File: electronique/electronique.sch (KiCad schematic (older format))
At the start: 35 parts, among them J1 Conn_02x07_Odd_Even, J10 PHOTOD3, J11 PHOTOD4, J12 Ultrason 3, J13 Moteur 2, J14 Moteur 1, J2 Conn_01x02, J3 Camera, J4 TOF1, J5 Conn_01x06, J6 Ultrason 1, J7 PHOTOD1, J8 PHOTOD2, J9 Ultrason 2, U1 STM32L451RETx, U2 LD1117S50TR_SOT223, U3 LD1117S33TR_SOT223, U4 LB1930MC-AH, U5 LB1930MC-AH, Y1 LFXTAL003240

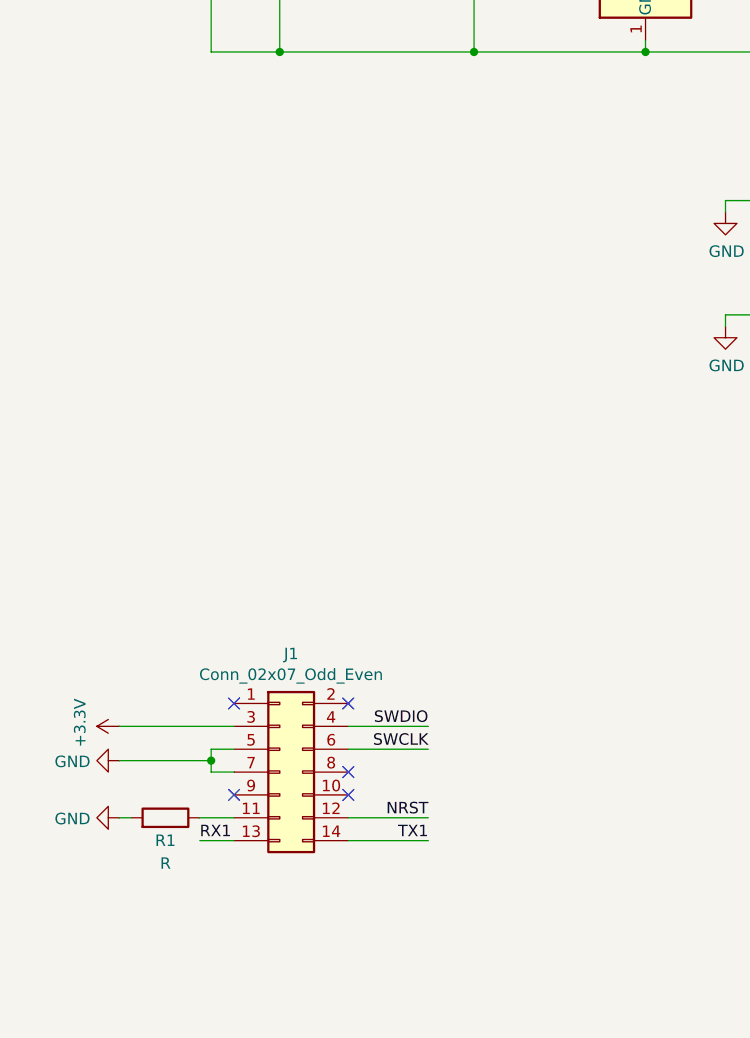
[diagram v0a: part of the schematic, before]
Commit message: Schema mis a jour pour la seance de projet
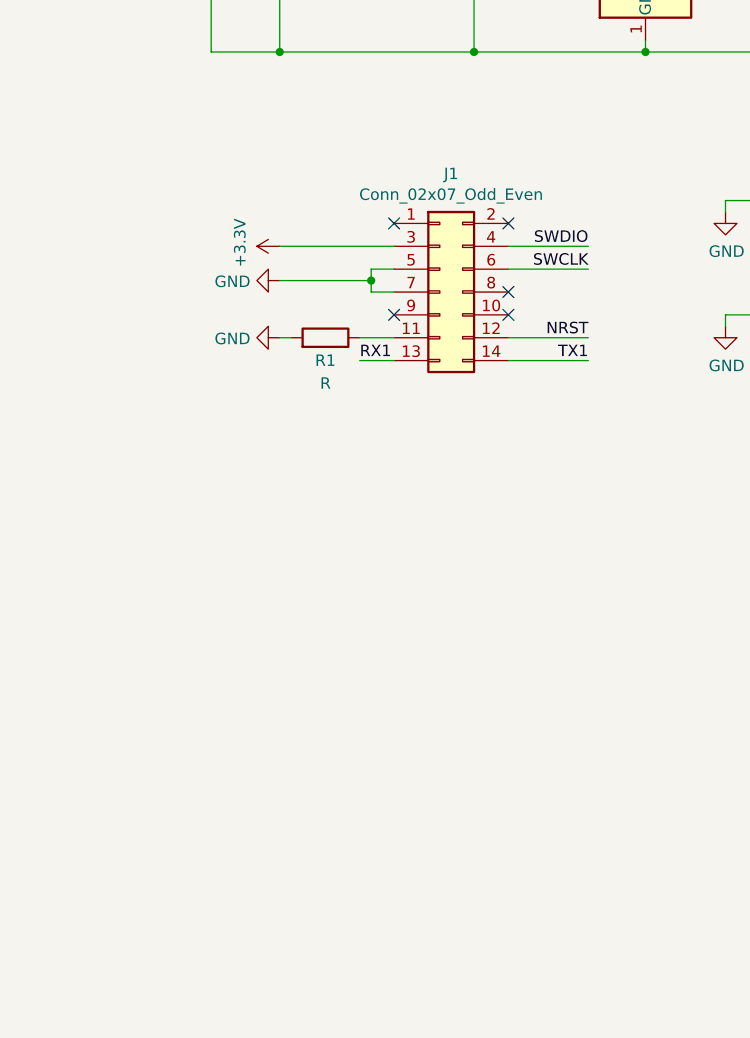
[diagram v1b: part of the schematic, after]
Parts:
- C1, C2: footprint (none) -> Capacitor_SMD:C_0805_2012Metric_Pad1.15x1.40mm_HandSolder
- R8, R9: footprint (none) -> Resistor_THT:R_Axial_DIN0207_L6.3mm_D2.5mm_P7.62mm_Horizontal
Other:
- moved on the sheet: J1, R1
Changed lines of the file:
@@
 EESchema Schematic File Version 4
-EELAYER 30 0
+LIBS:electronique-cache
+EELAYER 29 0
 EELAYER END
 $Descr A4 11693 8268
@@
 F 0 "C1" V 4052 2300 50  0000 C CNN
 F 1 "C" V 3961 2300 50  0000 C CNN
-F 2 "" H 3838 2150 50  0001 C CNN
+F 2 "Capacitor_SMD:C_0805_2012Metric_Pad1.15x1.40mm_HandSolder" H 3838 2150 50  0001 C CNN
 F 3 "~" H 3800 2300 50  0001 C CNN
 	1    3800 2300
@@
 F 0 "C2" V 3548 2800 50  0000 C CNN
 F 1 "C" V 3639 2800 50  0000 C CNN
-F 2 "" H 3838 2650 50  0001 C CNN
+F 2 "Capacitor_SMD:C_0805_2012Metric_Pad1.15x1.40mm_HandSolder" H 3838 2650 50  0001 C CNN
 F 3 "~" H 3800 2800 50  0001 C CNN
 	1    3800 2800
@@
 L Connector_Generic:Conn_02x07_Odd_Even J1
 U 1 1 615F66B1
-P 1550 4800
-F 0 "J1" H 1600 5317 50  0000 C CNN
-F 1 "Conn_02x07_Odd_Even" H 1600 5226 50  0000 C CNN
-F 2 "FTSH:SAMTEC_FTSH-107-01-L-DV-K-A" H 1550 4800 50  0001 C CNN
-F 3 "~" H 1550 4800 50  0001 C CNN
-	1    1550 4800
+P 2250 2700
+F 0 "J1" H 2300 3217 50  0000 C CNN
+F 1 "Conn_02x07_Odd_Even" H 2300 3126 50  0000 C CNN
+F 2 "FTSH:SAMTEC_FTSH-107-01-L-DV-K-A" H 2250 2700 50  0001 C CNN
+F 3 "~" H 2250 2700 50  0001 C CNN
+	1    2250 2700
 	1    0    0    -1
 $EndComp
@@
 	1    0    0    -1
 $EndComp
-NoConn ~ 1350 4500
-NoConn ~ 1850 4500
-NoConn ~ 1850 4800
-NoConn ~ 1850 4900
-NoConn ~ 1350 4900
+NoConn ~ 2050 2400
+NoConn ~ 2550 2400
+NoConn ~ 2550 2700
+NoConn ~ 2550 2800
+NoConn ~ 2050 2800
 $Comp
 L power:GND #PWR0106
 U 1 1 6161C108
-P 850 4750
-F 0 "#PWR0106" H 850 4500 50  0001 C CNN
-F 1 "GND" V 855 4622 50  0000 R CNN
-F 2 "" H 850 4750 50  0001 C CNN
-F 3 "" H 850 4750 50  0001 C CNN
-	1    850  4750
+P 1550 2650
+F 0 "#PWR0106" H 1550 2400 50  0001 C CNN
+F 1 "GND" V 1555 2522 50  0000 R CNN
+F 2 "" H 1550 2650 50  0001 C CNN
+F 3 "" H 1550 2650 50  0001 C CNN
+	1    1550 2650
 	0    1    1    0
 $EndComp
 Wire Wire Line
-	1350 4700 1250 4700
-Wire Wire Line
-	1250 4700 1250 4750
-Wire Wire Line
-	1250 4800 1350 4800
-Wire Wire Line
-	1250 4750 850  4750
-Connection ~ 1250 4750
-Wire Wire Line
-	1250 4750 1250 4800
+	2050 2600 1950 2600
+Wire Wire Line
+	1950 2600 1950 2650
+Wire Wire Line
+	1950 2700 2050 2700
+Wire Wire Line
+	1950 2650 1550 2650
+Connection ~ 1950 2650
+Wire Wire Line
+	1950 2650 1950 2700
 $Comp
 L power:GND #PWR0107
 U 1 1 6161D905
-P 850 5000
-F 0 "#PWR0107" H 850 4750 50  0001 C CNN
-F 1 "GND" V 855 4872 50  0000 R CNN
-F 2 "" H 850 5000 50  0001 C CNN
-F 3 "" H 850 5000 50  0001 C CNN
-	1    850  5000
+P 1550 2900
+F 0 "#PWR0107" H 1550 2650 50  0001 C CNN
+F 1 "GND" V 1555 2772 50  0000 R CNN
+F 2 "" H 1550 2900 50  0001 C CNN
+F 3 "" H 1550 2900 50  0001 C CNN
+	1    1550 2900
 	0    1    1    0
 $EndComp
@@
 L Device:R R1
 U 1 1 6161E3ED
-P 1050 5000
-F 0 "R1" V 950 5000 50  0000 C CNN
-F 1 "R" V 850 5000 50  0000 C CNN
-F 2 "Resistor_SMD:R_0805_2012Metric_Pad1.20x1.40mm_HandSolder" V 980 5000 50  0001 C CNN
-F 3 "~" H 1050 5000 50  0001 C CNN
-	1    1050 5000
+P 1750 2900
+F 0 "R1" V 1650 2900 50  0000 C CNN
+F 1 "R" V 1550 2900 50  0000 C CNN
+F 2 "Resistor_SMD:R_0805_2012Metric_Pad1.20x1.40mm_HandSolder" V 1680 2900 50  0001 C CNN
+F 3 "~" H 1750 2900 50  0001 C CNN
+	1    1750 2900
 	0    1    -1   0
 $EndComp
 Wire Wire Line
-	1200 5000 1350 5000
-Wire Wire Line
-	900  5000 850  5000
-Wire Wire Line
-	1850 4600 2200 4600
-Wire Wire Line
-	1850 4700 2200 4700
-Text Label 2200 4600 2    50   ~ 0
+	1900 2900 2050 2900
+Wire Wire Line
+	1600 2900 1550 2900
+Wire Wire Line
+	2550 2500 2900 2500
+Wire Wire Line
+	2550 2600 2900 2600
+Text Label 2900 2500 2    50   ~ 0
 SWDIO
-Text Label 2200 4700 2    50   ~ 0
+Text Label 2900 2600 2    50   ~ 0
 SWCLK
 Wire Wire Line
-	1850 5000 2200 5000
-Text Label 2200 5000 2    50   ~ 0
+	2550 2900 2900 2900
+Text Label 2900 2900 2    50   ~ 0
 NRST
 Wire Wire Line
-	1850 5100 2200 5100
-Text Label 2200 5100 2    50   ~ 0
+	2550 3000 2900 3000
+Text Label 2900 3000 2    50   ~ 0
 TX1
 Wire Wire Line
-	1350 5100 1200 5100
-Text Label 1200 5100 0    50   ~ 0
+	2050 3000 1900 3000
+Text Label 1900 3000 0    50   ~ 0
 RX1
 $Comp
 L power:+3.3V #PWR0108
 U 1 1 616474D0
-P 850 4600
-F 0 "#PWR0108" H 850 4450 50  0001 C CNN
-F 1 "+3.3V" H 865 4773 50  0000 C CNN
-F 2 "" H 850 4600 50  0001 C CNN
-F 3 "" H 850 4600 50  0001 C CNN
-	1    850  4600
+P 1550 2500
+F 0 "#PWR0108" H 1550 2350 50  0001 C CNN
+F 1 "+3.3V" H 1565 2673 50  0000 C CNN
+F 2 "" H 1550 2500 50  0001 C CNN
+F 3 "" H 1550 2500 50  0001 C CNN
+	1    1550 2500
 	0    -1   -1   0
 $EndComp
 Wire Wire Line
-	850  4600 1350 4600
+	1550 2500 2050 2500
 Text Label 6450 3000 2    50   ~ 0
 SWCLK
@@
 F 0 "R9" V 9443 1050 50  0000 C CNN
 F 1 "R" V 9534 1050 50  0000 C CNN
-F 2 "" V 9580 1050 50  0001 C CNN
+F 2 "Resistor_THT:R_Axial_DIN0207_L6.3mm_D2.5mm_P7.62mm_Horizontal" V 9580 1050 50  0001 C CNN
 F 3 "~" H 9650 1050 50  0001 C CNN
 	1    9650 1050
@@
 F 0 "R8" V 9393 2300 50  0000 C CNN
 F 1 "R" V 9484 2300 50  0000 C CNN
-F 2 "" V 9530 2300 50  0001 C CNN
+F 2 "Resistor_THT:R_Axial_DIN0207_L6.3mm_D2.5mm_P7.62mm_Horizontal" V 9530 2300 50  0001 C CNN
 F 3 "~" H 9600 2300 50  0001 C CNN
 	1    9600 2300
